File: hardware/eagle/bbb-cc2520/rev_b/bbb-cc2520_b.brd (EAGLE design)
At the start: 54.6 x 73.4 mm, 99 parts, among them J1 TC2030-IDC, J2 JUMPER-PTH-2-NO, P9/P8 BBB_HEADERS, U1 CC2520, U2 CC2520, U3 CAT24C256WI-GT3, U4 CC2591, U5 CD4051B-53B, U6 NRF51822QF, X1 NX2520SA, X2 NX2520SA, X3 16MHz

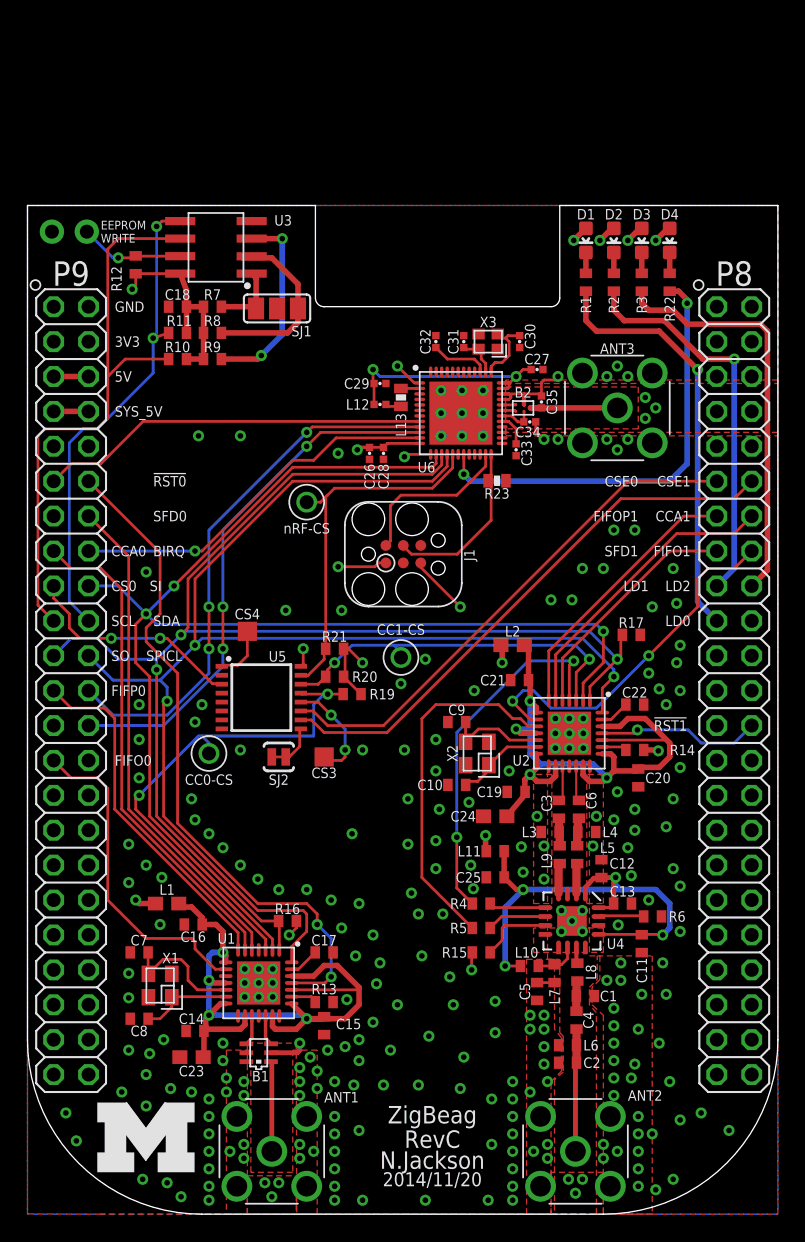
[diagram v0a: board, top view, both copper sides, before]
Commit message: restore rev b
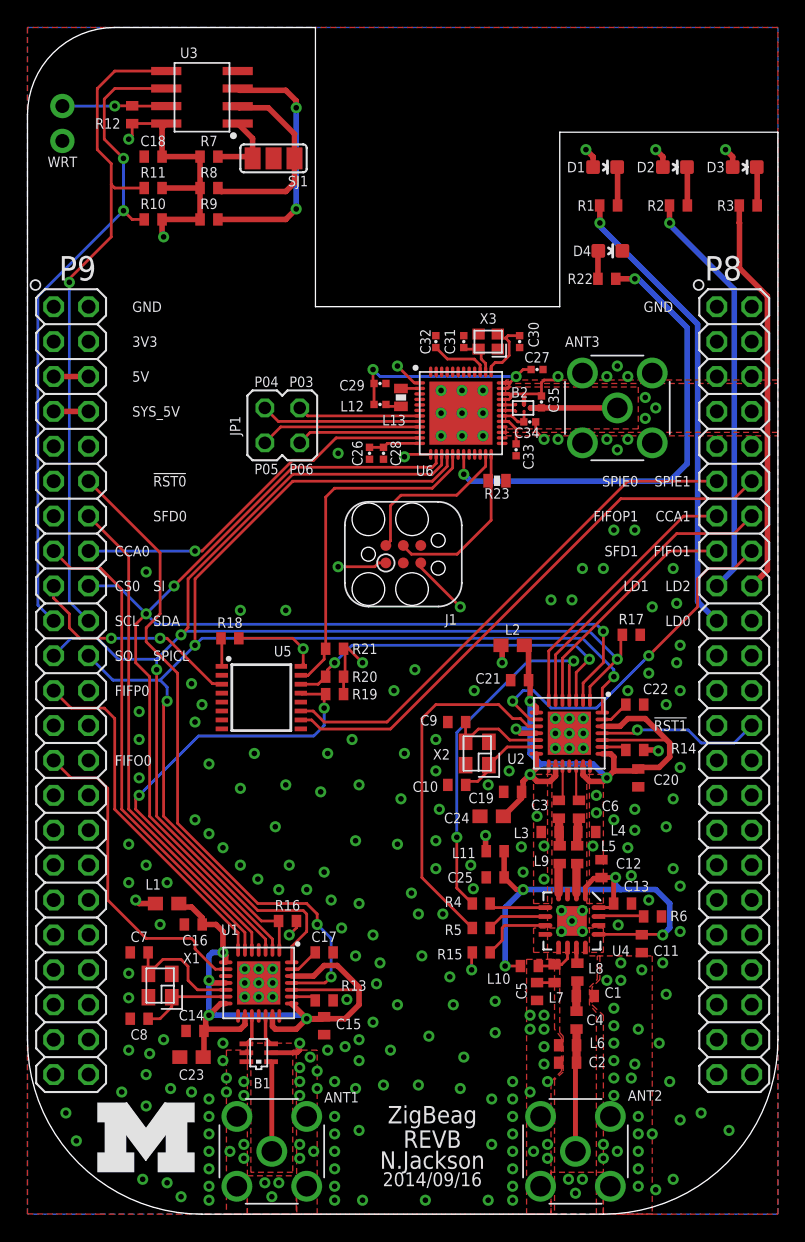
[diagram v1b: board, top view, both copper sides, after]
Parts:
- removed CS0, CS1, CS2: TEST_POINT_0.040IN, headers:TESTPOINT_0.040IN
- removed CS3, CS4: TPTP14SQ, testpad:TP14SQ
- removed J2: JUMPER-PTH-2-NO, SparkFun-Passives:PTH-JUMPER-2-NO_NO_SILK
- removed SJ2: JUMPER-PAD-2-NC_BY_TRACE, SparkFun-Passives:PAD-JUMPER-2-NC_BY_TRACE_YES_SILK
- added JP1: (no value), jumper:JP2Q
- added R18: 10k 1%, rcl:R0402
- added WRT: JUMPER-PTH-2-NO, SparkFun-Passives:PTH-JUMPER-2-NO_NO_SILK
- moved C18 11.1 mm to (9.14, 77.0)
- moved U3 11.0 mm to (12.7, 81.3)
- moved R12 10.9 mm to (7.62, 80.0)
- moved R7 10.9 mm to (13.2, 77.0)
- moved SJ1 10.9 mm to (17.9, 76.8)
- moved R11 10.7 mm to (9.14, 74.7)
- moved R8 10.5 mm to (13.2, 74.7)
- moved R10 10.3 mm to (9.14, 72.4)
- moved R9 10.2 mm to (13.2, 72.4)
- moved R3 9.55 mm to (52.5, 73.4), turned to 0 degrees
- moved D3 9.20 mm to (52.2, 76.2), turned to 270 degrees
- moved R2 7.30 mm to (47.4, 73.4), turned to 0 degrees
- moved D2 6.94 mm to (47.1, 76.2), turned to 270 degrees
- moved R1 5.83 mm to (42.3, 73.4), turned to 0 degrees
- moved D1 5.51 mm to (42.0, 76.2), turned to 270 degrees
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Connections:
- net CSE0 renamed SPIE0
- net CSE1 renamed SPIE1
- removed net !RESET2: P9/P8.P9_11, U6.8
- removed net N$65: SJ2.1, U5.9
- removed net N$66: CS3.TP, U5.12
- removed net N$67: CS4.TP, U5.1
- removed net UARTRX: P9/P8.P9_24, U6.9
- removed net UARTTX: P9/P8.P9_26, U6.10
- new net CS3: U5.12
- new net CS4: R18.1, U5.1
- new net CS5: U5.5
- new net CS6: U5.2
- new net CS7: U5.4
- new net P04: JP1.2, U6.8
- new net P05: JP1.4, U6.9
- new net P06: JP1.3, U6.10
- net CS0: no longer CS0.TESTPOINT
- net CS1: no longer CS1.TESTPOINT
- net CS2: no longer CS2.TESTPOINT
- net GND: now also D4.C, U5.9, WRT.2; no longer J2.2, SJ2.2
- net N$31: now also WRT.1; no longer J2.1
- net N$63: now also D4.A, R22.1; no longer D4.C, R22.2
- net N$64: now also R22.2; no longer R22.1
- net P03: now also JP1.1
- net VCC: now also R18.2; no longer D4.A
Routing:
- net UARTRX: track 39.6 -> 0.00 mm, vias 3 -> 0
- net UARTTX: track 38.7 -> 0.00 mm, vias 3 -> 0
- net !RESET2: track 28.4 -> 0.00 mm
- net SDA: track 35.6 -> 49.0 mm, vias 2 -> 1
- net P05: track 0.00 -> 11.8 mm
- net P04: track 0.00 -> 11.7 mm
- net P06: track 0.00 -> 9.04 mm
- net P03: track 0.00 -> 8.97 mm
- net N$66: track 7.80 -> 0.00 mm, vias 2 -> 0
- net VCC: track 43.8 -> 51.5 mm, vias 14 -> 13
- net SCL: track 42.4 -> 48.2 mm, vias 0 -> 2
- net N$32: track 14.4 -> 18.5 mm
- net N$67: track 3.96 -> 0.00 mm
- net LED0: track 30.6 -> 33.8 mm
- net N$64: track 31.9 -> 35.0 mm
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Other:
- board size 54.6 x 73.4 mm -> 54.6 x 86.4 mm
- board text added: "2014/09/16"
- board text added: "P03"
- board text added: "P04"
- board text added: "P05"
- board text added: "P06"
- board text added: "REVB"
- board text added: "SPIE0"
- board text added: "SPIE1"
- board text removed: "2014/11/20"
- board text removed: "BIRQ"
- board text removed: "CC0-CS"
- board text removed: "CC1-CS"
- board text removed: "CSE0"
- board text removed: "CSE1"
- board text removed: "EEPROM WRITE"
- board text removed: "RevC"
- board text removed: "nRF-CS"
